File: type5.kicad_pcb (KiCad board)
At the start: 2 copper layers, 83.8 x 57.5 mm, 3 parts, among them P1 CONN_01X09, P2 CONN_01X26, U1 TEENSYPP2

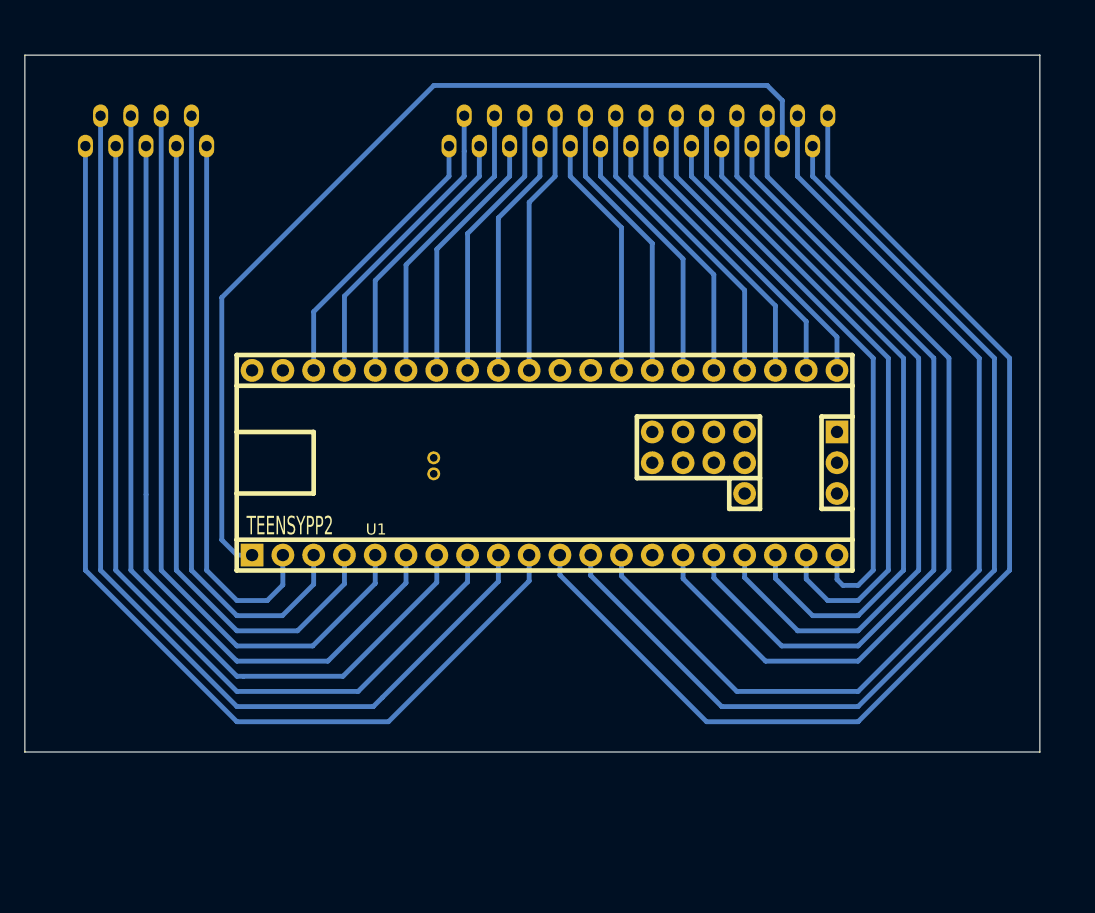
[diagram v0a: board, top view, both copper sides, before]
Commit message: new pcb
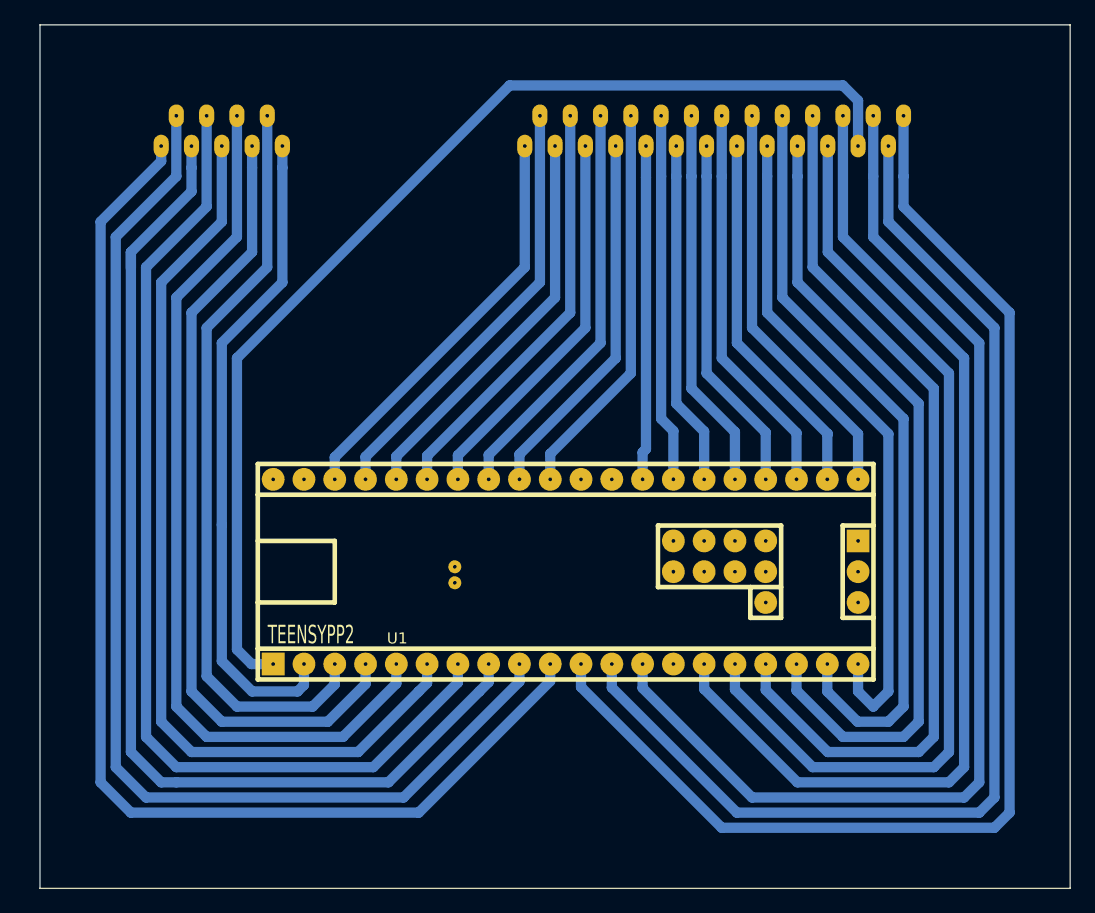
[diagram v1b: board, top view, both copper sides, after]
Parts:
- U1: footprint myfootprint:TEENSYPP2 -> myfootprint:TEENSYPP2_mod
- moved U1 9.16 mm to (144.6, 105.1)
- moved P1 6.25 mm to (116.2, 71.2)
- moved P2 6.25 mm to (156.2, 72.5)
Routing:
- net Net-(P1-Pad1): track 83.7 -> 98.6 mm
- net Net-(P1-Pad3): track 74.1 -> 88.9 mm
- net Net-(P1-Pad2): track 81.4 -> 95.6 mm
- net Net-(P1-Pad4): track 71.8 -> 84.5 mm
- net Net-(P1-Pad5): track 64.5 -> 76.5 mm
- net Net-(P2-Pad22): track 73.5 -> 85.1 mm
- net Net-(P2-Pad23): track 80.8 -> 92.4 mm
- net Net-(P1-Pad6): track 62.2 -> 73.4 mm
- net Net-(P2-Pad26): track 92.7 -> 103.7 mm
- net Net-(P2-Pad21): track 66.2 -> 77.1 mm
- net Net-(P2-Pad5): track 21.0 -> 31.9 mm
- net Net-(P2-Pad8): track 21.9 -> 32.8 mm
- net Net-(P2-Pad1): track 23.1 -> 34.0 mm
- net Net-(P2-Pad7): track 19.9 -> 30.8 mm
- net Net-(P2-Pad6): track 23.0 -> 33.8 mm
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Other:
- board size 83.8 x 57.5 mm -> 85 x 71.2 mm
- net class Default: clearance 0.15 -> 0.1; trace_width 0.4 -> 0.85
- rule trace_clearance: 0.15 -> 0.1
